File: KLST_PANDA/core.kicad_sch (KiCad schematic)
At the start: 34 parts, among them SW1 BUTTON_RESET, SW2 BUTTON_BOOT_FLASH, U2 STM32H723ZGTx, Y1 16MHz

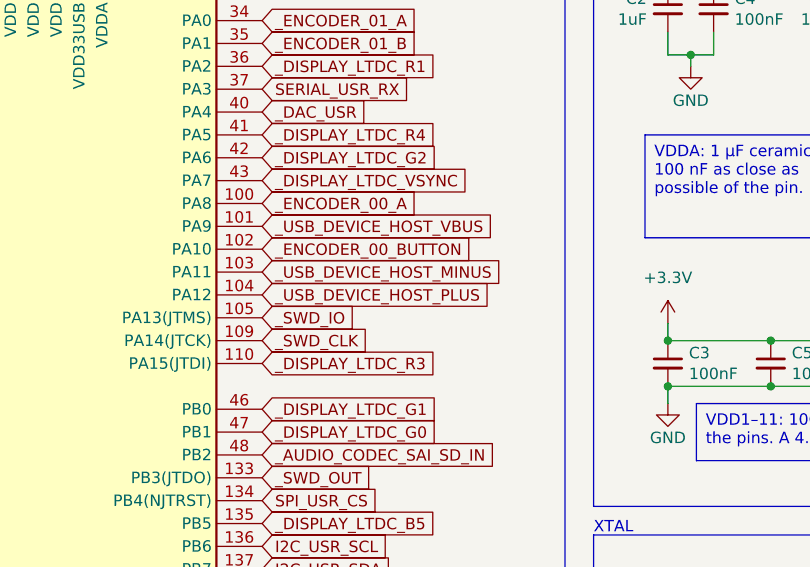
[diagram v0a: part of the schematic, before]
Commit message: continued routing
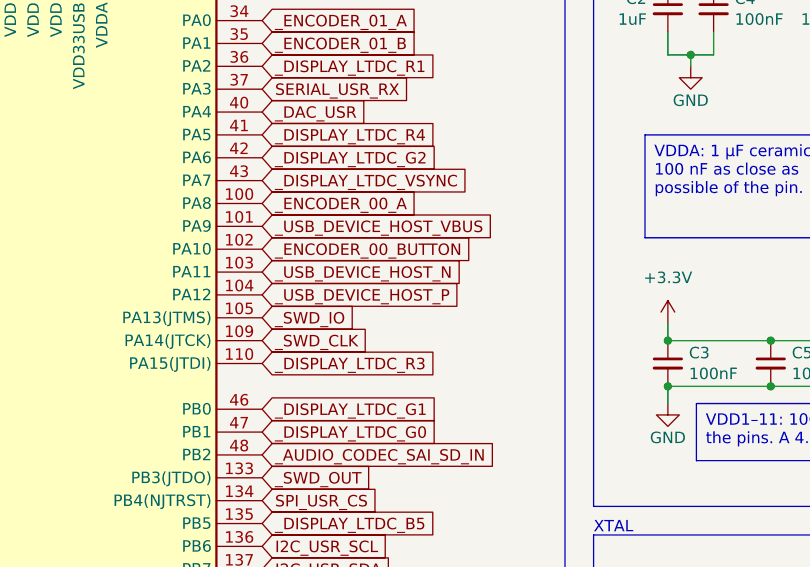
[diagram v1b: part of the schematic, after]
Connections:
- net _USB_DEVICE_HOST_MINUS renamed _USB_DEVICE_HOST_N
- net _USB_DEVICE_HOST_PLUS renamed _USB_DEVICE_HOST_P
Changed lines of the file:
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@@
     )
   )
-  (global_label "_USB_DEVICE_HOST_PLUS" (shape input) (at 119.38 67.31 0) (fields_autoplaced)
+  (global_label "_USB_DEVICE_HOST_P" (shape input) (at 119.38 67.31 0) (fields_autoplaced)
     (effects (font (size 1.27 1.27)) (justify left))
     (property "Intersheetrefs" "${INTERSHEET_REFS}" (at 146.2532 67.31 0)
@@
     )
   )
-  (global_label "_USB_DEVICE_HOST_MINUS" (shape input) (at 119.38 64.77 0) (fields_autoplaced)
+  (global_label "_USB_DEVICE_HOST_N" (shape input) (at 119.38 64.77 0) (fields_autoplaced)
     (effects (font (size 1.27 1.27)) (justify left))
     (property "Intersheetrefs" "${INTERSHEET_REFS}" (at 147.3418 64.77 0)
